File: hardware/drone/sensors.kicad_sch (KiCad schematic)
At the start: 4 parts, among them U14 ICM-42688-P

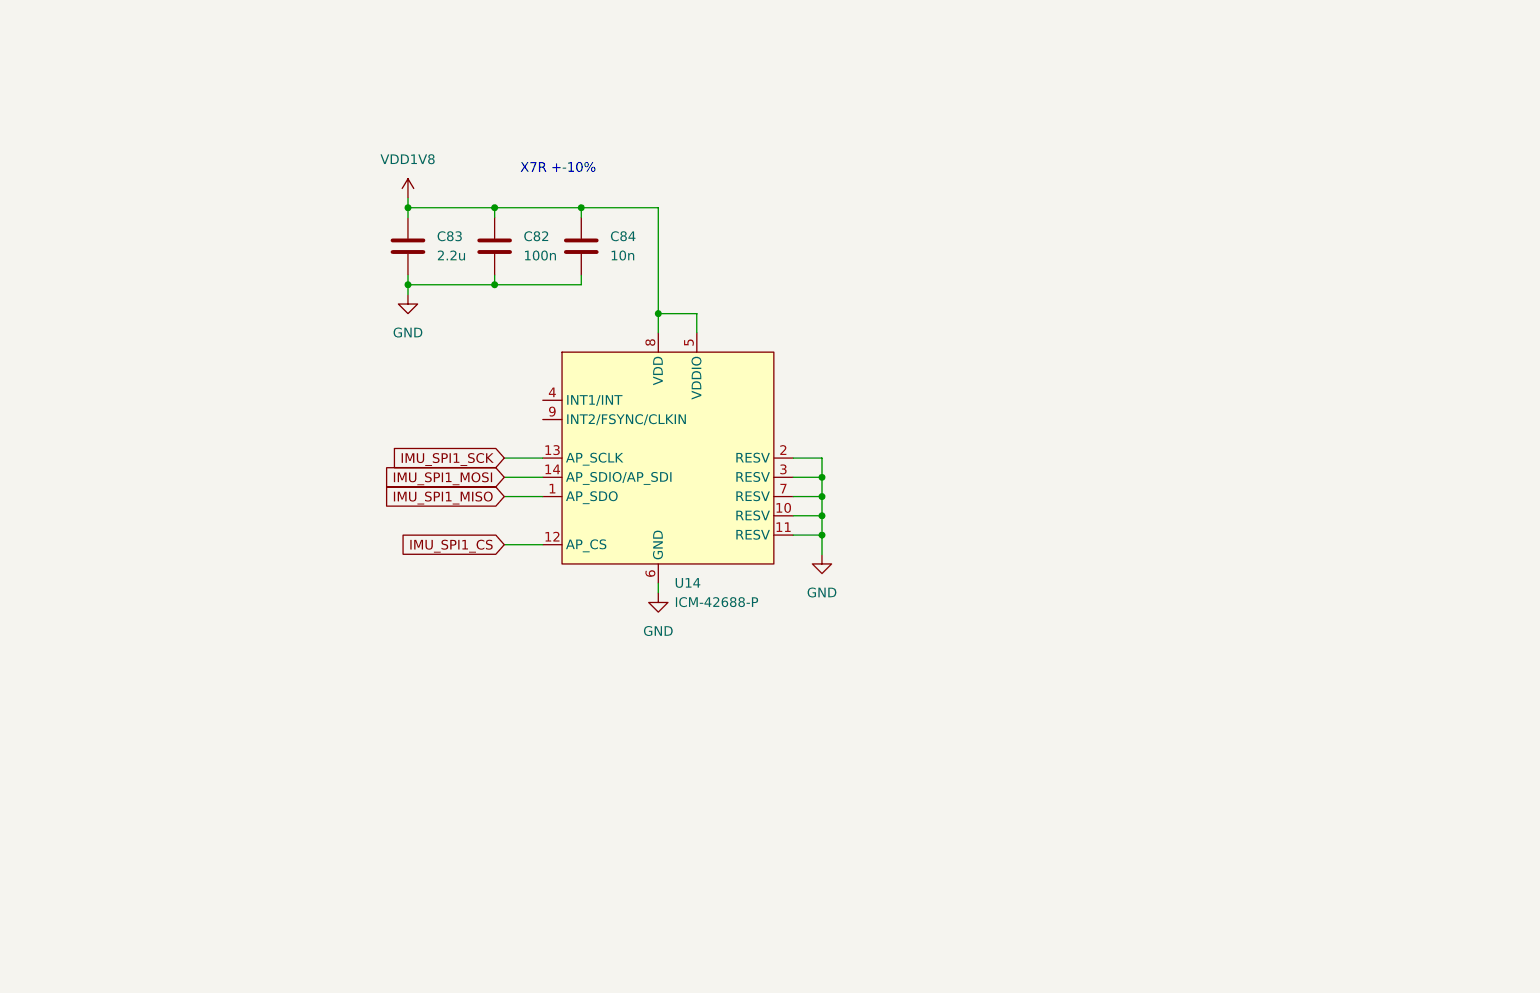
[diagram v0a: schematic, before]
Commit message: Finished GNSS, did more pinmuxxing
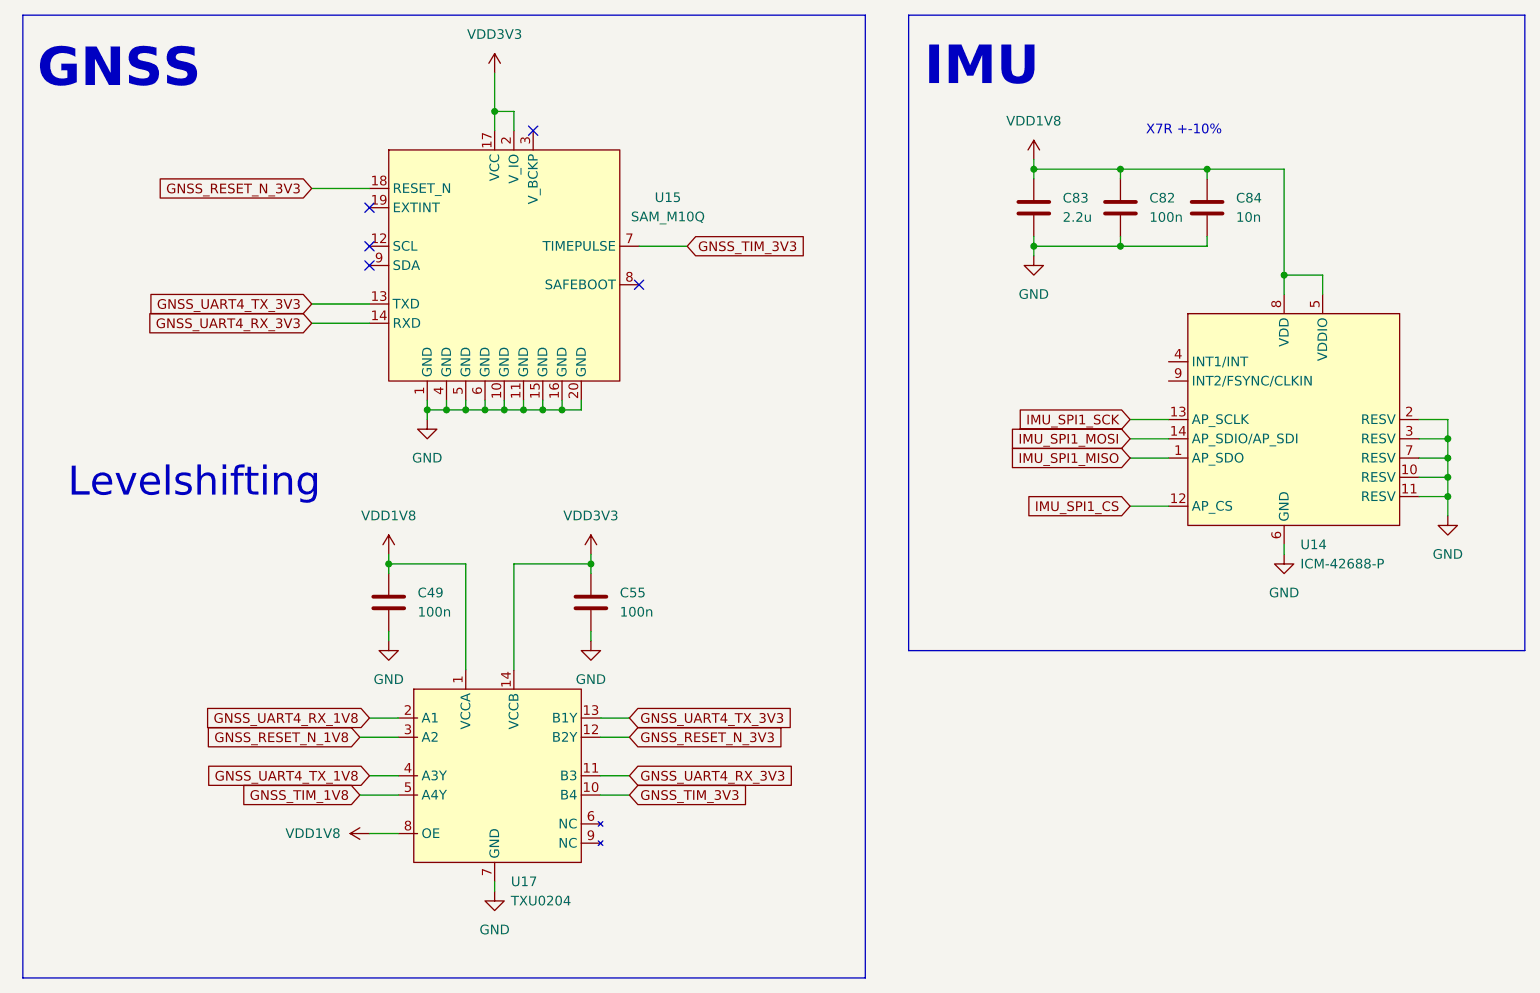
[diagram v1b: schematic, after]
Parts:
- added C49, C55: 100n, symbol Device:C
- added U15: SAM_M10Q, Package_LGA:LGA-16_3x3mm_P0.5mm_LayoutBorder3x5y, symbol SoftDrone:SAM_M10Q
- added U17: TXU0204, symbol SoftDrone:TXU0204
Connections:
- net GND: now also C49.2, C55.2, U15.1 (GND), U15.10 (GND), U15.11 (GND), U15.15 (GND), U15.16 (GND), U15.20 (GND), U15.4 (GND), U15.5 (GND), U15.6 (GND), U17.7 (GND)
- net VDD1V8: now also C49.1, U17.1 (VCCA), U17.8 (OE)
- new net GNSS_RESET_N_1V8: U17.3 (A2)
- new net GNSS_RESET_N_3V3: U15.18 (RESET_N), U17.12 (B2Y)
- new net GNSS_TIM_1V8: U17.5 (A4Y)
- new net GNSS_TIM_3V3: U15.7 (TIMEPULSE), U17.10 (B4)
- new net GNSS_UART4_RX_1V8: U17.2 (A1)
- new net GNSS_UART4_RX_3V3: U15.14 (RXD), U17.11 (B3)
- new net GNSS_UART4_TX_1V8: U17.4 (A3Y)
- new net GNSS_UART4_TX_3V3: U15.13 (TXD), U17.13 (B1Y)
- new net VDD3V3: C55.1, U15.17 (VCC), U15.2 (V_IO), U17.14 (VCCB)
- no-connect marks 0 -> 5
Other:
- note added: "GNSS"
- note added: "IMU"
- note added: "Levelshifting"
- moved on the sheet: C82, C83, C84, U14
